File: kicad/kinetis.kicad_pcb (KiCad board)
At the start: 2 copper layers, 88.9 x 88.9 mm, 75 parts, among them J1 USB_Micro_B, J2 JLink_SWD_20pin, J3 CONN_01X16, J4 CONN_01X16, J5 FTDI_Connector, J6 CONN_01X16, J7 CONN_01X16, M1 #4-40 Mounting Hole, M2 #4-40 Mounting Hole, M3 #4-40 Mounting Hole, M4 #4-40 Mounting Hole, SW1 DPDT, SW2 SPST, SW3 SPST, SW4 SPST, SW5 SPST, SW6 SPST, U1 LM1117-ADJ, U2 MKL16Z64VLH4, Y1 12.000 MHz

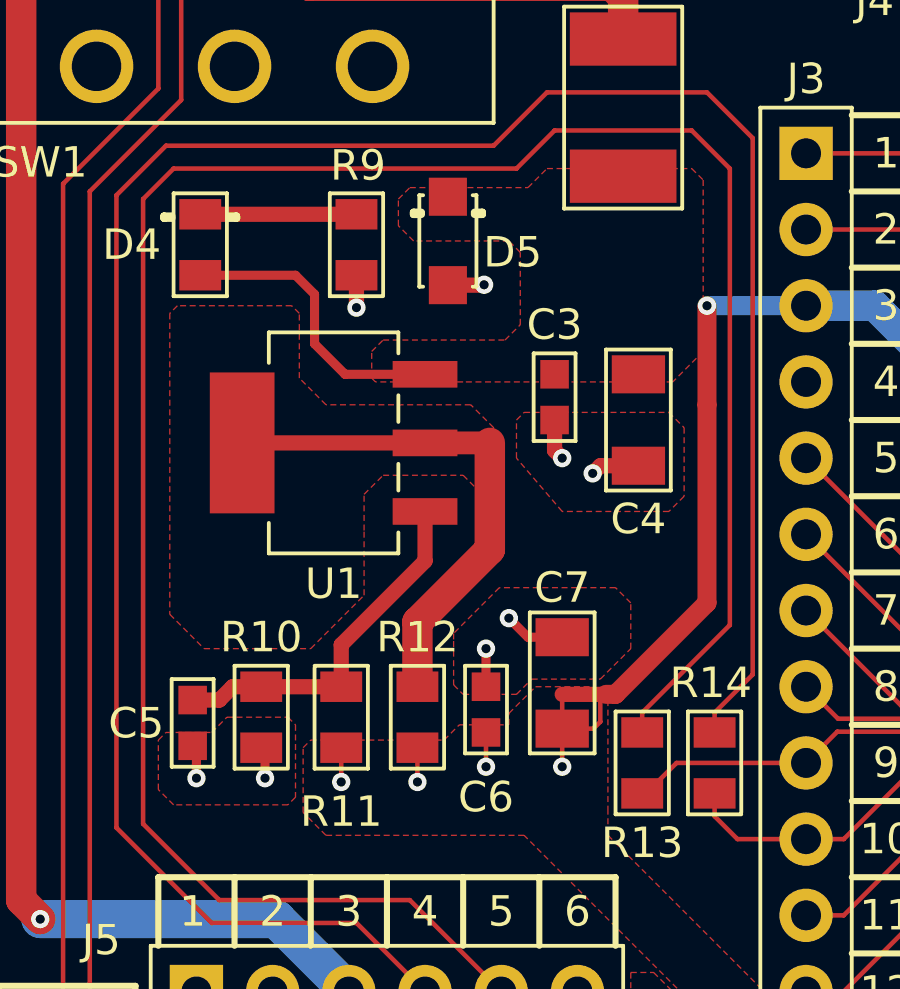
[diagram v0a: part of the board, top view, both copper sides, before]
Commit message: Yet more tweaks
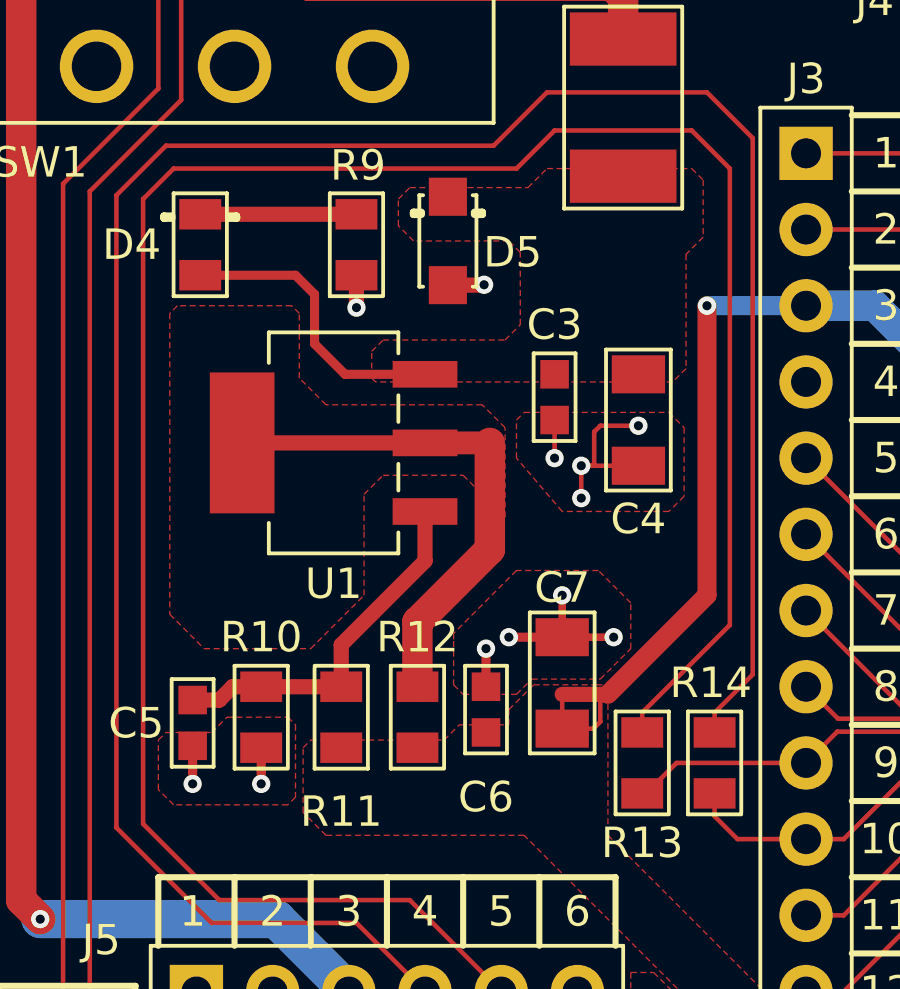
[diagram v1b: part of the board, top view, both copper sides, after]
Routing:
- net GND: track 124.7 -> 132.4 mm, vias 37 -> 41
- net +3.3V: track 329.2 -> 324.0 mm, vias 11 -> 7
